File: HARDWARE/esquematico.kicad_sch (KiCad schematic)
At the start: 52 parts, among them J1 Screw_Terminal_01x02, J10 LCD I2C, J12 Screw_Terminal_01x02, J13 Screw_Terminal_01x02, J14 Screw_Terminal_01x02, J15 Screw_Terminal_01x02, J2 Screw_Terminal_01x02, J3 Screw_Terminal_01x02, J4 Screw_Terminal_01x02, J5 Screw_Terminal_01x02, J6 PINERA, Q1 2N7000, Q2 2N7000, Q3 2N7000, Q4 2N7000, U1 PC817, U2 ESP32-DEVKITC-32D, U3 L7805, U4 PC817, U5 PC817, U6 PC817

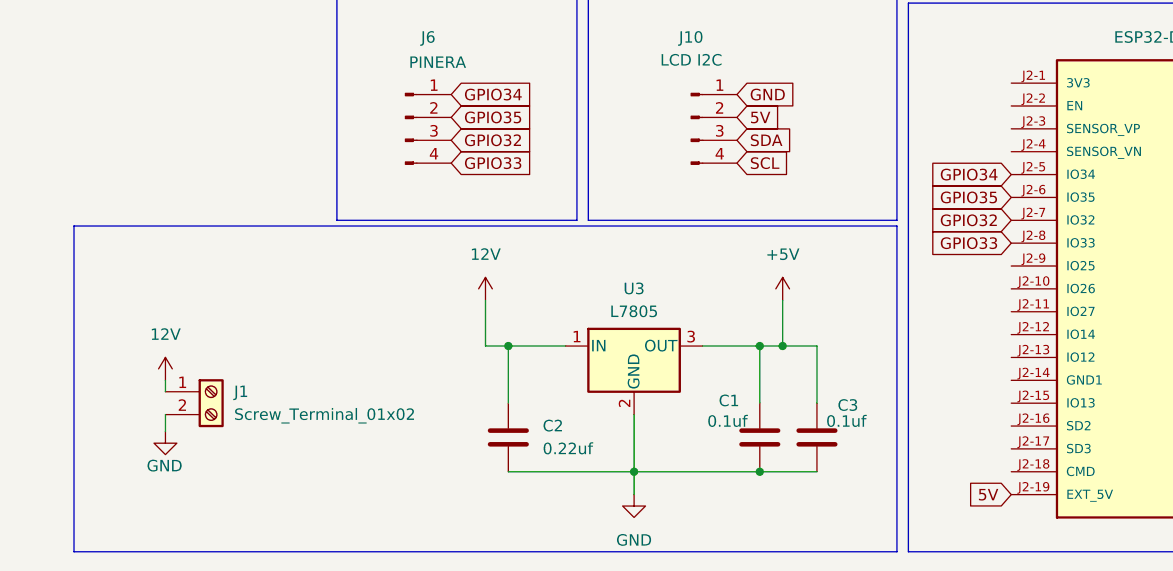
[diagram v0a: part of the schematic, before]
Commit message: termine de corregir la placa
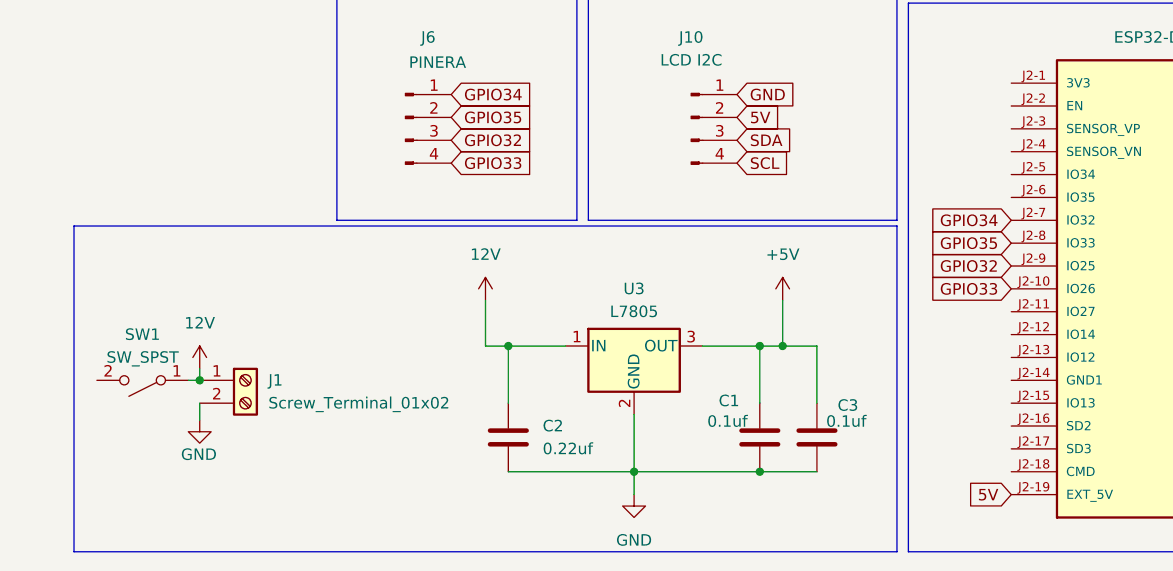
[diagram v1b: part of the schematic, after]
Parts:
- added SW1: SW_SPST, Connector_PinHeader_2.54mm:PinHeader_1x02_P2.54mm_Vertical, symbol Switch:SW_SPST
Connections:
- net 12V: now also SW1.1 (A)
- net GPIO32: now also U2.J2-9 (IO25); no longer U2.J2-7 (IO32)
- net GPIO33: now also U2.J2-10 (IO26); no longer U2.J2-8 (IO33)
- net GPIO34: now also U2.J2-7 (IO32); no longer U2.J2-5 (IO34)
- net GPIO35: now also U2.J2-8 (IO33); no longer U2.J2-6 (IO35)
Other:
- moved on the sheet: J1
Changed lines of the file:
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@@
 	)
 	(junction
+		(at 31.75 176.53)
+		(diameter 0)
+		(color 0 0 0 0)
+	)
+	(junction
 		(at 93.98 186.69)
 		(diameter 0)
@@
 	(wire
 		(pts
-			(xy 27.94 177.8) (xy 27.94 176.53)
+			(xy 31.75 176.53) (xy 31.75 175.26)
 		)
 		(stroke
@@
 	(wire
 		(pts
-			(xy 27.94 180.34) (xy 27.94 182.245)
+			(xy 31.75 179.07) (xy 31.75 180.975)
 		)
 		(stroke
@@
 	(wire
 		(pts
+			(xy 30.48 176.53) (xy 31.75 176.53)
+		)
+		(stroke
+			(width 0)
+			(type default)
+		)
+	)
+	(wire
+		(pts
 			(xy 73.025 59.69) (xy 73.025 63.5)
 		)
@@
 	(global_label "GPIO35"
 		(shape input)
-		(at 121.92 156.21 180)
+		(at 121.92 161.29 180)
 		(fields_autoplaced yes)
 		(effects
@@
 		)
 		(property "Intersheetrefs" "${INTERSHEET_REFS}"
-			(at 112.0405 156.21 0)
+			(at 112.0405 161.29 0)
 			(effects
 				(font
@@
 	(global_label "GPIO33"
 		(shape input)
-		(at 121.92 161.29 180)
+		(at 121.92 166.37 180)
 		(fields_autoplaced yes)
 		(effects
@@
 		)
 		(property "Intersheetrefs" "${INTERSHEET_REFS}"
-			(at 112.0405 161.29 0)
+			(at 112.0405 166.37 0)
 			(effects
 				(font
@@
 	(global_label "GPIO32"
 		(shape input)
-		(at 121.92 158.75 180)
+		(at 121.92 163.83 180)
 		(fields_autoplaced yes)
 		(effects
@@
 		)
 		(property "Intersheetrefs" "${INTERSHEET_REFS}"
-			(at 112.0405 158.75 0)
+			(at 112.0405 163.83 0)
 			(effects
 				(font
@@
 	(global_label "GPIO34"
 		(shape input)
-		(at 121.92 153.67 180)
+		(at 121.92 158.75 180)
 		(fields_autoplaced yes)
 		(effects
@@
 		)
 		(property "Intersheetrefs" "${INTERSHEET_REFS}"
-			(at 112.0405 153.67 0)
+			(at 112.0405 158.75 0)
 			(effects
 				(font
@@
 	)
 	(symbol
+		(lib_id "Switch:SW_SPST")
+		(at 25.4 176.53 180)
+		(unit 1)
+		(exclude_from_sim no)
+		(in_bom yes)
+		(on_board yes)
+		(dnp no)
+		(fields_autoplaced yes)
+		(property "Reference" "SW1"
+			(at 25.4 171.45 0)
+			(effects
+				(font
+					(size 1.27 1.27)
+				)
+			)
+		)
+		(property "Value" "SW_SPST"
+			(at 25.4 173.99 0)
+			(effects
+				(font
+					(size 1.27 1.27)
+				)
+			)
+		)
+		(property "Footprint" "Connector_PinHeader_2.54mm:PinHeader_1x02_P2.54mm_Vertical"
+			(at 25.4 176.53 0)
+			(effects
+				(font
+					(size 1.27 1.27)
+				)
+				(hide yes)
+			)
+		)
+		(property "Datasheet" "~"
+			(at 25.4 176.53 0)
+			(effects
+				(font
+					(size 1.27 1.27)
+				)
+				(hide yes)
+			)
+		)
+		(property "Description" "Single Pole Single Throw (SPST) switch"
+			(at 25.4 176.53 0)
+			(effects
+				(font
+					(size 1.27 1.27)
+				)
+				(hide yes)
+			)
+		)
+		(pin "2"
+		)
+		(pin "1"
+		)
+		(instances
+			(project ""
+				(path "/3fb1f07d-b939-40dd-b220-aa81ef24414e"
+					(reference "SW1")
+					(unit 1)
+				)
+			)
+		)
+	)
+	(symbol
 		(lib_id "Transistor_FET:2N7000")
 		(at 67.945 113.03 0)
@@
 	(symbol
 		(lib_id "power:VCC")
-		(at 27.94 176.53 0)
+		(at 31.75 175.26 0)
 		(unit 1)
 		(exclude_from_sim no)
@@
 		(fields_autoplaced yes)
 		(property "Reference" "#PWR08"
-			(at 27.94 180.34 0)
+			(at 31.75 179.07 0)
 			(effects
 				(font
@@
 		)
 		(property "Value" "12V"
-			(at 27.94 171.45 0)
+			(at 31.75 170.18 0)
 			(effects
 				(font
@@
 		)
 		(property "Footprint" ""
-			(at 27.94 176.53 0)
+			(at 31.75 175.26 0)
 			(effects
 				(font
@@
 		)
 		(property "Datasheet" ""
-			(at 27.94 176.53 0)
+			(at 31.75 175.26 0)
 			(effects
 				(font
@@
 		)
 		(property "Description" "Power symbol creates a global label with name \"VCC\""
-			(at 27.94 176.53 0)
+			(at 31.75 175.26 0)
 			(effects
 				(font
@@
 	(symbol
 		(lib_id "power:GND")
-		(at 27.94 182.245 0)
+		(at 31.75 180.975 0)
 		(unit 1)
 		(exclude_from_sim no)
@@
 		(dnp no)
 		(property "Reference" "#PWR07"
-			(at 27.94 188.595 0)
+			(at 31.75 187.325 0)
 			(effects
 				(font
@@
 		)
 		(property "Value" "GND"
-			(at 29.845 186.055 0)
+			(at 33.655 184.785 0)
 			(effects
 				(font
@@
 		)
 		(property "Footprint" ""
-			(at 27.94 182.245 0)
+			(at 31.75 180.975 0)
 			(effects
 				(font
@@
 		)
 		(property "Datasheet" ""
-			(at 27.94 182.245 0)
+			(at 31.75 180.975 0)
 			(effects
 				(font
@@
 		)
 		(property "Description" "Power symbol creates a global label with name \"GND\" , ground"
-			(at 27.94 182.245 0)
+			(at 31.75 180.975 0)
 			(effects
 				(font
@@
 	(symbol
 		(lib_id "Connector:Screw_Terminal_01x02")
-		(at 33.02 177.8 0)
+		(at 36.83 176.53 0)
 		(unit 1)
 		(exclude_from_sim no)
@@
 		(fields_autoplaced yes)
 		(property "Reference" "J1"
-			(at 35.56 177.7999 0)
+			(at 39.37 176.5299 0)
 			(effects
 				(font
@@
 		)
 		(property "Value" "Screw_Terminal_01x02"
-			(at 35.56 180.3399 0)
+			(at 39.37 179.0699 0)
 			(effects
 				(font
@@
 		)
 		(property "Footprint" "TerminalBlock:TerminalBlock_bornier-2_P5.08mm"
-			(at 33.02 177.8 0)
+			(at 36.83 176.53 0)
 			(effects
 				(font
@@
 		)
 		(property "Datasheet" "~"
-			(at 33.02 177.8 0)
+			(at 36.83 176.53 0)
 			(effects
 				(font
@@
 		)
 		(property "Description" "Generic screw terminal, single row, 01x02, script generated (kicad-library-utils/schlib/autogen/connector/)"
-			(at 33.02 177.8 0)
+			(at 36.83 176.53 0)
 			(effects
 				(font
